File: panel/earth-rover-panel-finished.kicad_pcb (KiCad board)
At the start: 2 copper layers, 226.1 x 115.6 mm, 138 parts, among them J1 Conn_01x04_Male, J1 Conn_02x04_Male_UnitPerRow, J10 Connector:Screw_Terminal_01x02, J2 Conn_01x04_Male, J3 Conn_01x04_Male, J3 Conn_02x03_Male, J4 Conn_01x04_Male, J4 Conn_02x03_Male, J5 5.4mm/2.5mm, J5 Conn_02x03_Male, J6 Conn_02x03_Male, J7 Conn_01x03_Male, J8 Conn_01x03_Male, J9 Conn_02x06_Male_UnitPerRow, Q1 BC517, SW1 SW_Push, SW1 SW_SPST, SW2 SW_Push, SW3 SW_DPDT_x2, U1 NRF24L01+, U1 TLE4905L, U1 Teensy3.2, U2 NRF24L01+ breakout, U2 TLE4905L, U2 Teensy3.2, U3 LM2940CT-5.0, U3 ULN2803A, U4 MIC29502WT

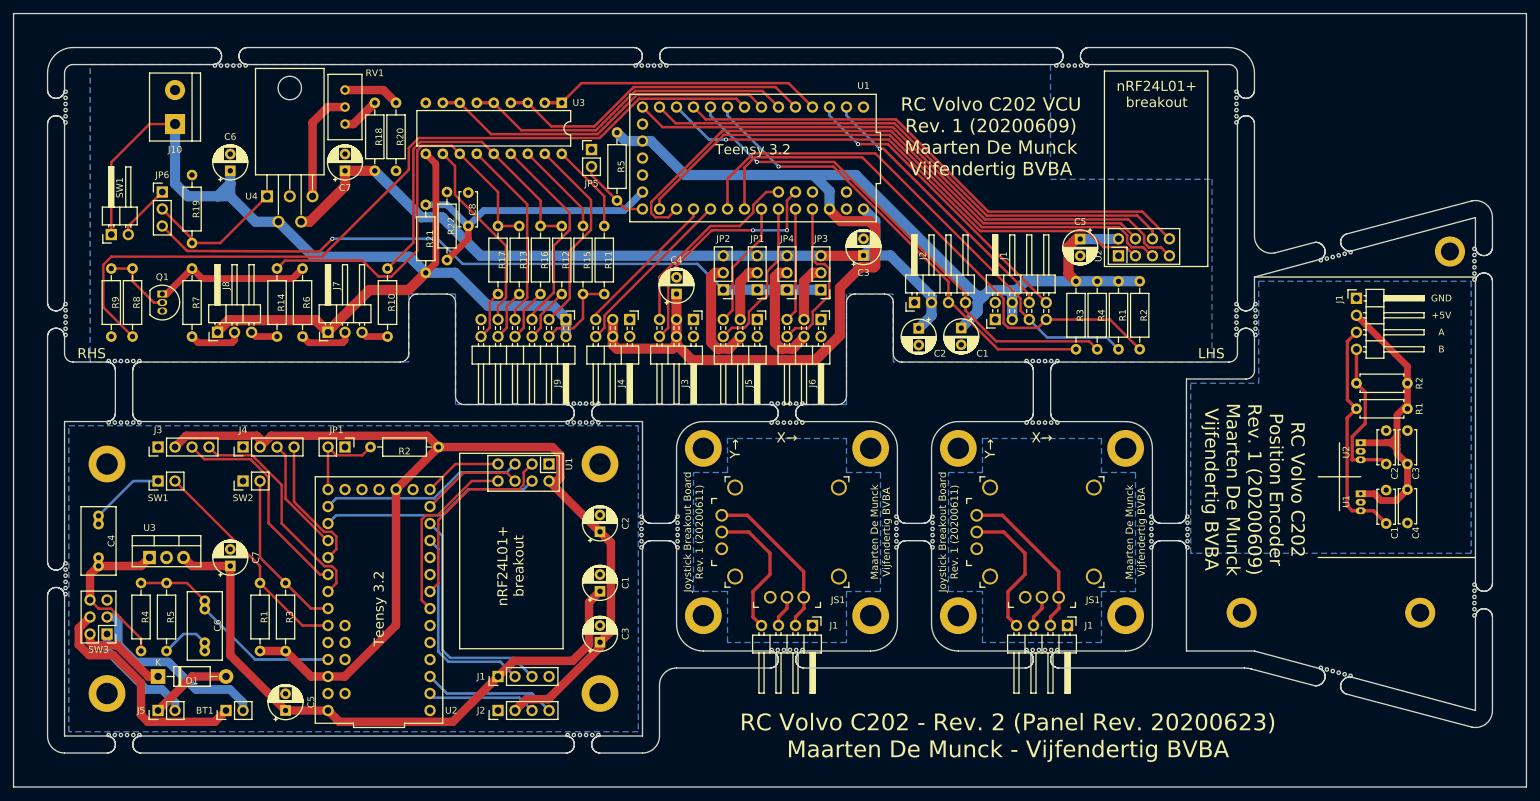
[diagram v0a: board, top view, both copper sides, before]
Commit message: Update panel to KiCad 6.0
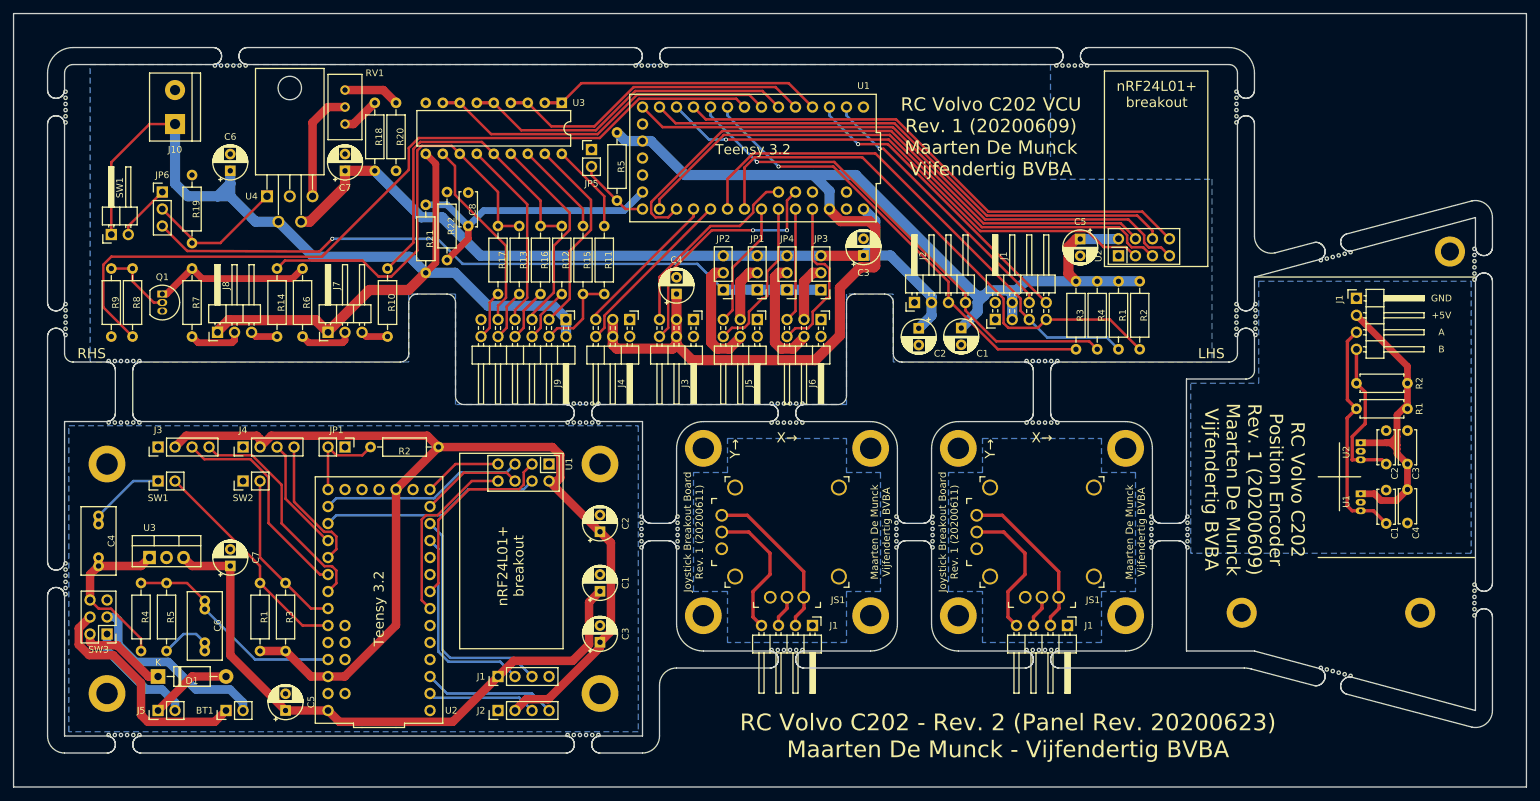
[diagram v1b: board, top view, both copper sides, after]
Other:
- net class Default removed
